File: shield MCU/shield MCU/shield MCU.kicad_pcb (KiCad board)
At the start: 2 copper layers, 16 parts, among them J1 IR_sensor, J2 IR_sensor, J3 IR_sensor, J4 IR_sensor, J5 IR_sensor, J6 BATT, SW1 Pwr_Sw, U1 pwr_mgr_1, U3 gy50, U4 NUCLEO144-F429ZI

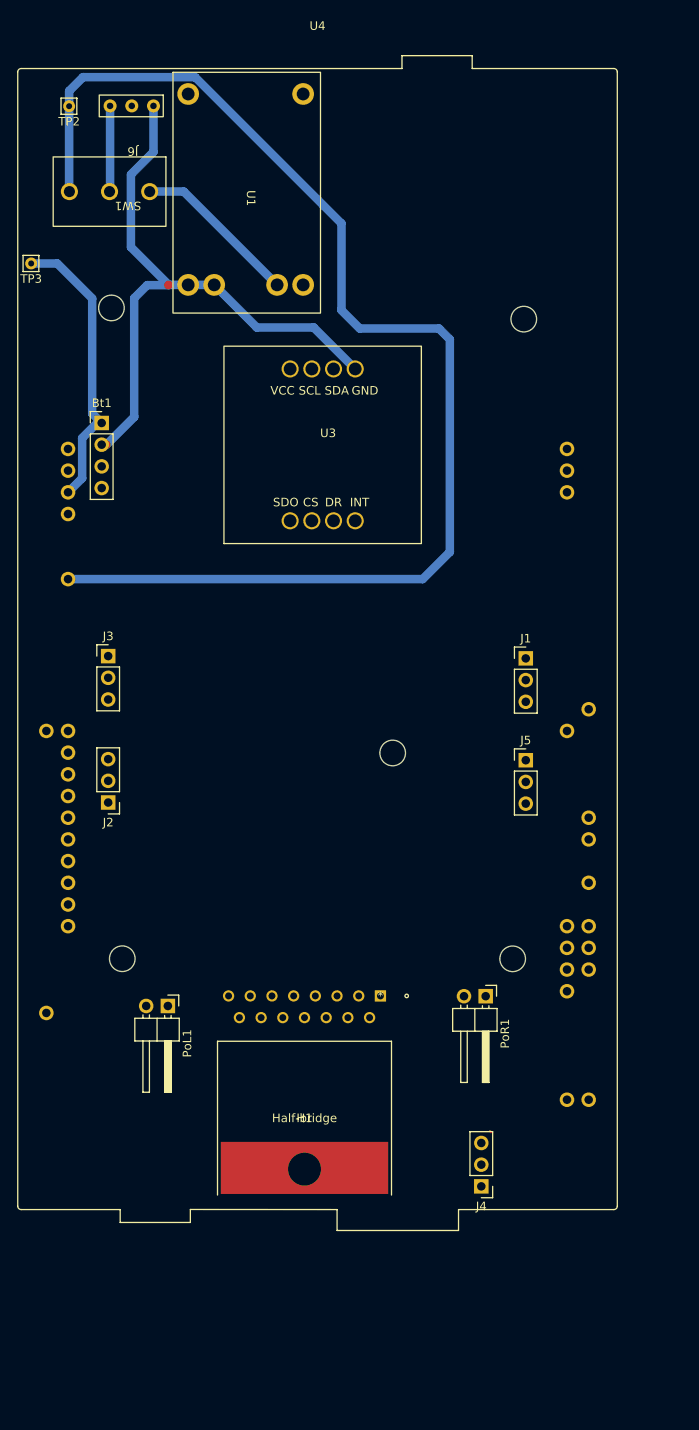
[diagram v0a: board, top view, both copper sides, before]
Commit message: PCB layout done
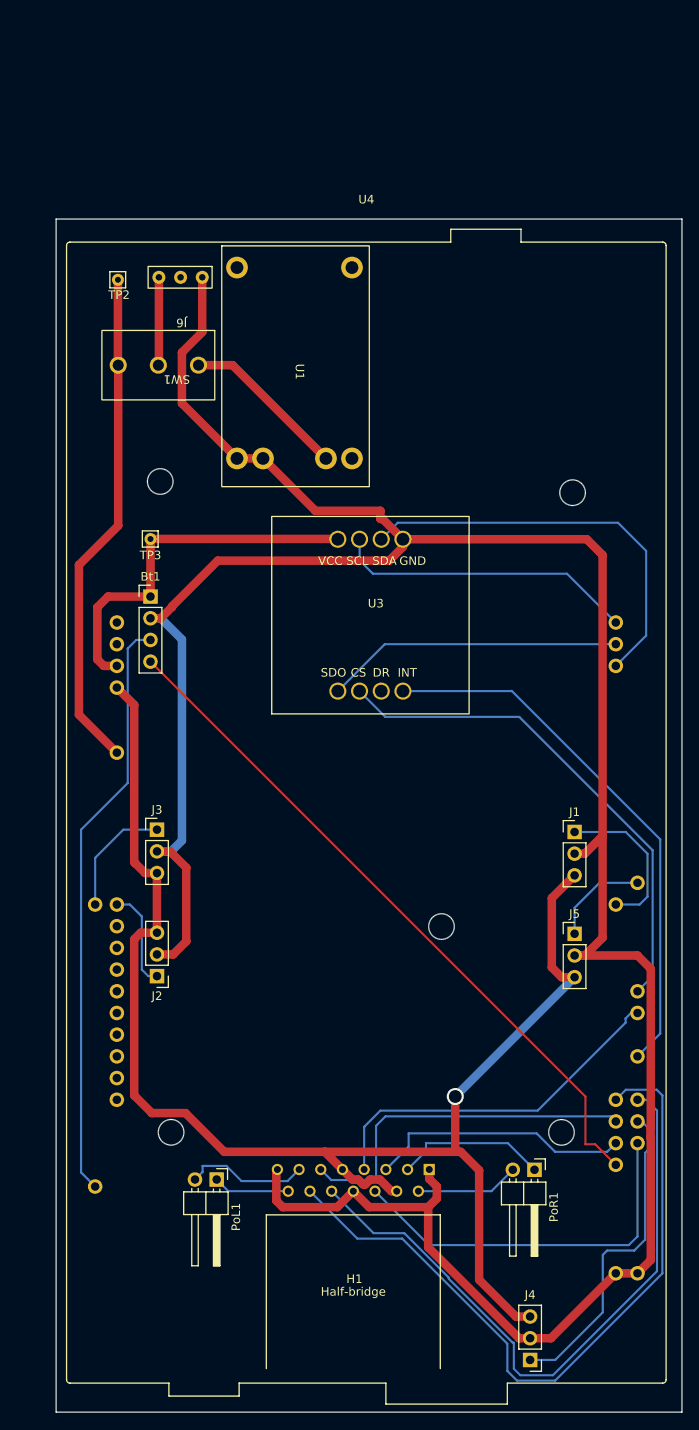
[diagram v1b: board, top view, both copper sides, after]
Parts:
- moved TP3 35.2 mm to (105.2, 70.2)
- moved J2 21.1 mm to (105.9, 121.4)
- moved J4 21.1 mm to (149.6, 166.4)
- moved PoL1 21.1 mm to (112.9, 145.2)
- moved PoR1 21.1 mm to (150.1, 144.1)
- moved H1 21.1 mm to (137.8, 144.1)
- moved J1 21.1 mm to (154.8, 104.5)
- moved J5 21.1 mm to (154.8, 116.5)
- moved TP2 21.1 mm to (101.3, 39.9)
- moved U1 21.1 mm to (113.5, 35.9)
- moved U4 21.1 mm to (98.7, 67.3)
- moved SW1 21.1 mm to (112.7, 45.8)
- moved Bt1 21.1 mm to (105.2, 77.0)
- moved J3 21.1 mm to (105.9, 104.3)
- moved J6 20.9 mm to (112.4, 38.3)
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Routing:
- net GND: track 73.5 -> 319.8 mm
- net /5V: track 0.00 -> 169.4 mm, vias 0 -> 1
- net /Vin: track 146.6 -> 59.1 mm
- net Net-(H1-Pad12): track 0.00 -> 84.6 mm
- net Net-(Bt1-Pad4): track 0.00 -> 82.2 mm
- net Net-(H1-Pad10): track 0.00 -> 75.5 mm
- net Net-(Bt1-Pad3): track 0.00 -> 69.0 mm
- net Net-(U3-Pad4): track 0.00 -> 63.9 mm
- net Net-(U3-Pad2): track 0.00 -> 59.3 mm
- net Net-(U3-Pad7): track 0.00 -> 48.1 mm
- net Net-(H1-Pad6): track 0.00 -> 44.7 mm
- net Net-(H1-Pad7): track 0.00 -> 42.8 mm
- net Net-(H1-Pad11): track 0.00 -> 41.9 mm
- net Net-(J4-Pad1): track 0.00 -> 38.2 mm
- net Net-(U3-Pad6): track 0.00 -> 35.6 mm
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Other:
- board outline added: 73.3 x 139.7 mm
